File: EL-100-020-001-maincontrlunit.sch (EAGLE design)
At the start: 186 parts, among them T1 WS-TST-90°, U1 VNI4140K-32, U16 24AA256-I/SN, U19 ABS10-32.768KHZ-7-T, U2 VNI4140K-32, U3 VNI4140K-32, U8 MCP7940N-I/SN, U9 PMEG2005ET, X1 944-12-46-00, X10 S2L3.50/8/90G, X11 S2L3.50/8/90G, X12 S2L3.50/8/90G, X13 140-08-FLACHBAND1.27, X14 944-12-2-00, X2 944-12-46-00, X3 90G-14, X4 90G-14, X5 Q-063209, X6 Q-063209, X7 Q-063209, X8 Q-063209, X9 S2L3.50/8/90G

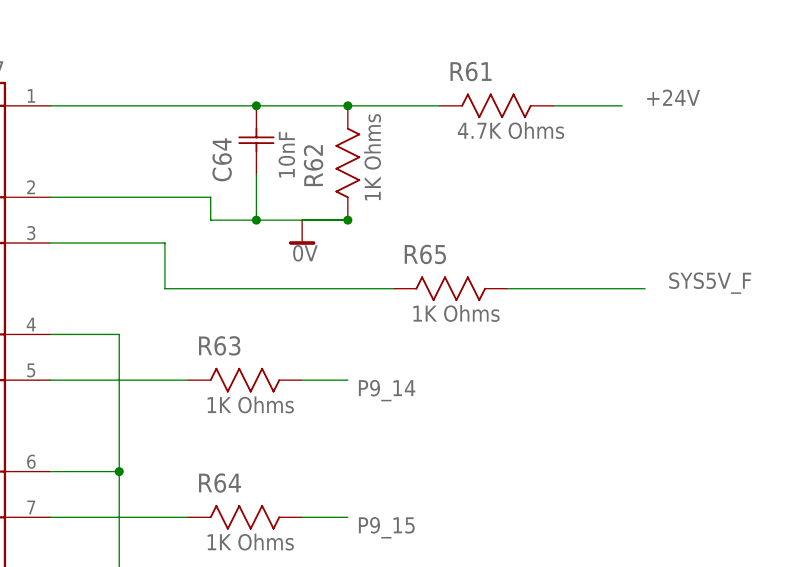
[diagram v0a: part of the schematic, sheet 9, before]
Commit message: Din rail
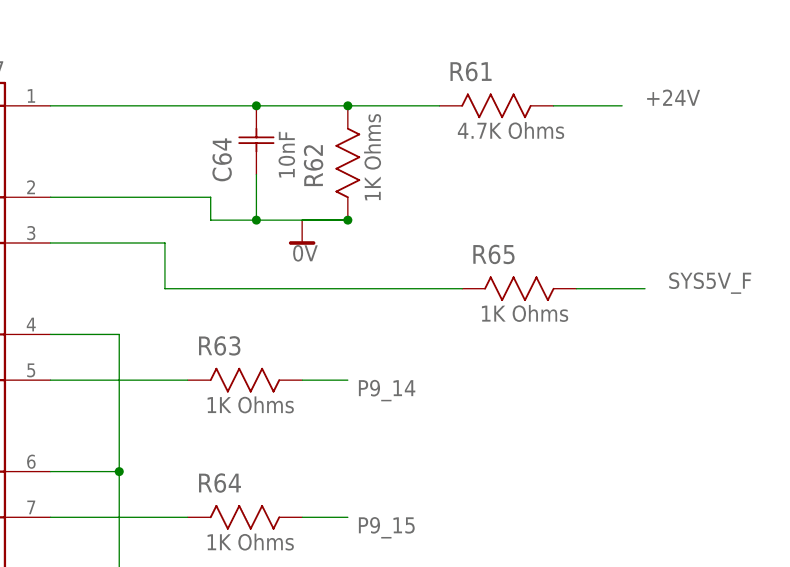
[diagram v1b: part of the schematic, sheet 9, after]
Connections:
- net VADC_1.8V: now also X5.B10
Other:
- moved on the sheet: R65
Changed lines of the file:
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@@
 <label x="350.52" y="193.04" size="1.778" layer="95"/>
 <pinref part="R69" gate="A" pin="2"/>
-<wire x1="317.5" y1="193.04" x2="271.78" y2="193.04" width="0.1524" layer="91"/>
+<wire x1="317.5" y1="193.04" x2="254" y2="193.04" width="0.1524" layer="91"/>
 <wire x1="317.5" y1="205.74" x2="317.5" y2="193.04" width="0.1524" layer="91"/>
 <junction x="317.5" y="193.04"/>
@@
 </segment>
 <segment>
-<wire x1="271.78" y1="190.5" x2="327.66" y2="190.5" width="0.1524" layer="91"/>
 <label x="350.52" y="190.5" size="1.778" layer="95"/>
 <pinref part="R70" gate="A" pin="2"/>
+<wire x1="246.38" y1="190.5" x2="327.66" y2="190.5" width="0.1524" layer="91"/>
 <wire x1="327.66" y1="190.5" x2="347.98" y2="190.5" width="0.1524" layer="91"/>
 <wire x1="327.66" y1="205.74" x2="327.66" y2="190.5" width="0.1524" layer="91"/>
@@
 </segment>
 <segment>
-<wire x1="271.78" y1="195.58" x2="304.8" y2="195.58" width="0.1524" layer="91"/>
 <label x="350.52" y="195.58" size="1.778" layer="95"/>
 <pinref part="R68" gate="A" pin="2"/>
+<wire x1="264.16" y1="195.58" x2="304.8" y2="195.58" width="0.1524" layer="91"/>
 <wire x1="304.8" y1="195.58" x2="347.98" y2="195.58" width="0.1524" layer="91"/>
 <wire x1="304.8" y1="205.74" x2="304.8" y2="195.58" width="0.1524" layer="91"/>
@@
 </segment>
 </net>
+<net name="VADC_1.8V" class="0">
+<segment>
+<pinref part="X5" gate="G$1" pin="B10"/>
+<wire x1="157.48" y1="180.34" x2="165.1" y2="180.34" width="0.1524" layer="91"/>
+<label x="165.1" y="180.34" size="1.778" layer="95"/>
+</segment>
+</net>
 </nets>
 </sheet>
@@
 </instance>
 <instance part="SUPPLY106" gate="G$1" x="213.36" y="139.7"/>
-<instance part="R65" gate="A" x="243.84" y="182.88" smashed="yes">
-<attribute name="VALUE" x="245.7958" y="179.2224" size="1.778" layer="96" ratio="10" rot="SR0"/>
-<attribute name="NAME" x="244.8306" y="185.6486" size="2.0828" layer="95" ratio="10" rot="SR0"/>
-<attribute name="MF" x="243.84" y="182.88" size="1.778" layer="96" rot="R270" display="off"/>
+<instance part="R65" gate="A" x="251.46" y="182.88" smashed="yes">
+<attribute name="VALUE" x="253.4158" y="179.2224" size="1.778" layer="96" ratio="10" rot="SR0"/>
+<attribute name="NAME" x="252.4506" y="185.6486" size="2.0828" layer="95" ratio="10" rot="SR0"/>
+<attribute name="MF" x="251.46" y="182.88" size="1.778" layer="96" rot="R270" display="off"/>
 </instance>
 <instance part="X13" gate="G$1" x="66.04" y="180.34" smashed="yes">
@@
 <wire x1="205.74" y1="187.96" x2="218.44" y2="187.96" width="0.1524" layer="91"/>
 <wire x1="218.44" y1="187.96" x2="218.44" y2="182.88" width="0.1524" layer="91"/>
-<wire x1="218.44" y1="182.88" x2="243.84" y2="182.88" width="0.1524" layer="91"/>
+<wire x1="218.44" y1="182.88" x2="251.46" y2="182.88" width="0.1524" layer="91"/>
 <pinref part="R65" gate="A" pin="2"/>
 </segment>
@@
 <segment>
 <pinref part="R65" gate="A" pin="1"/>
-<wire x1="256.54" y1="182.88" x2="271.78" y2="182.88" width="0.1524" layer="91"/>
+<wire x1="264.16" y1="182.88" x2="271.78" y2="182.88" width="0.1524" layer="91"/>
 <label x="274.32" y="182.88" size="1.778" layer="95"/>
 </segment>
